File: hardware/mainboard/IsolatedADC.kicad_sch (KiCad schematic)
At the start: 22 parts, among them IC4 ADC 24bit, IC5 LTC1799

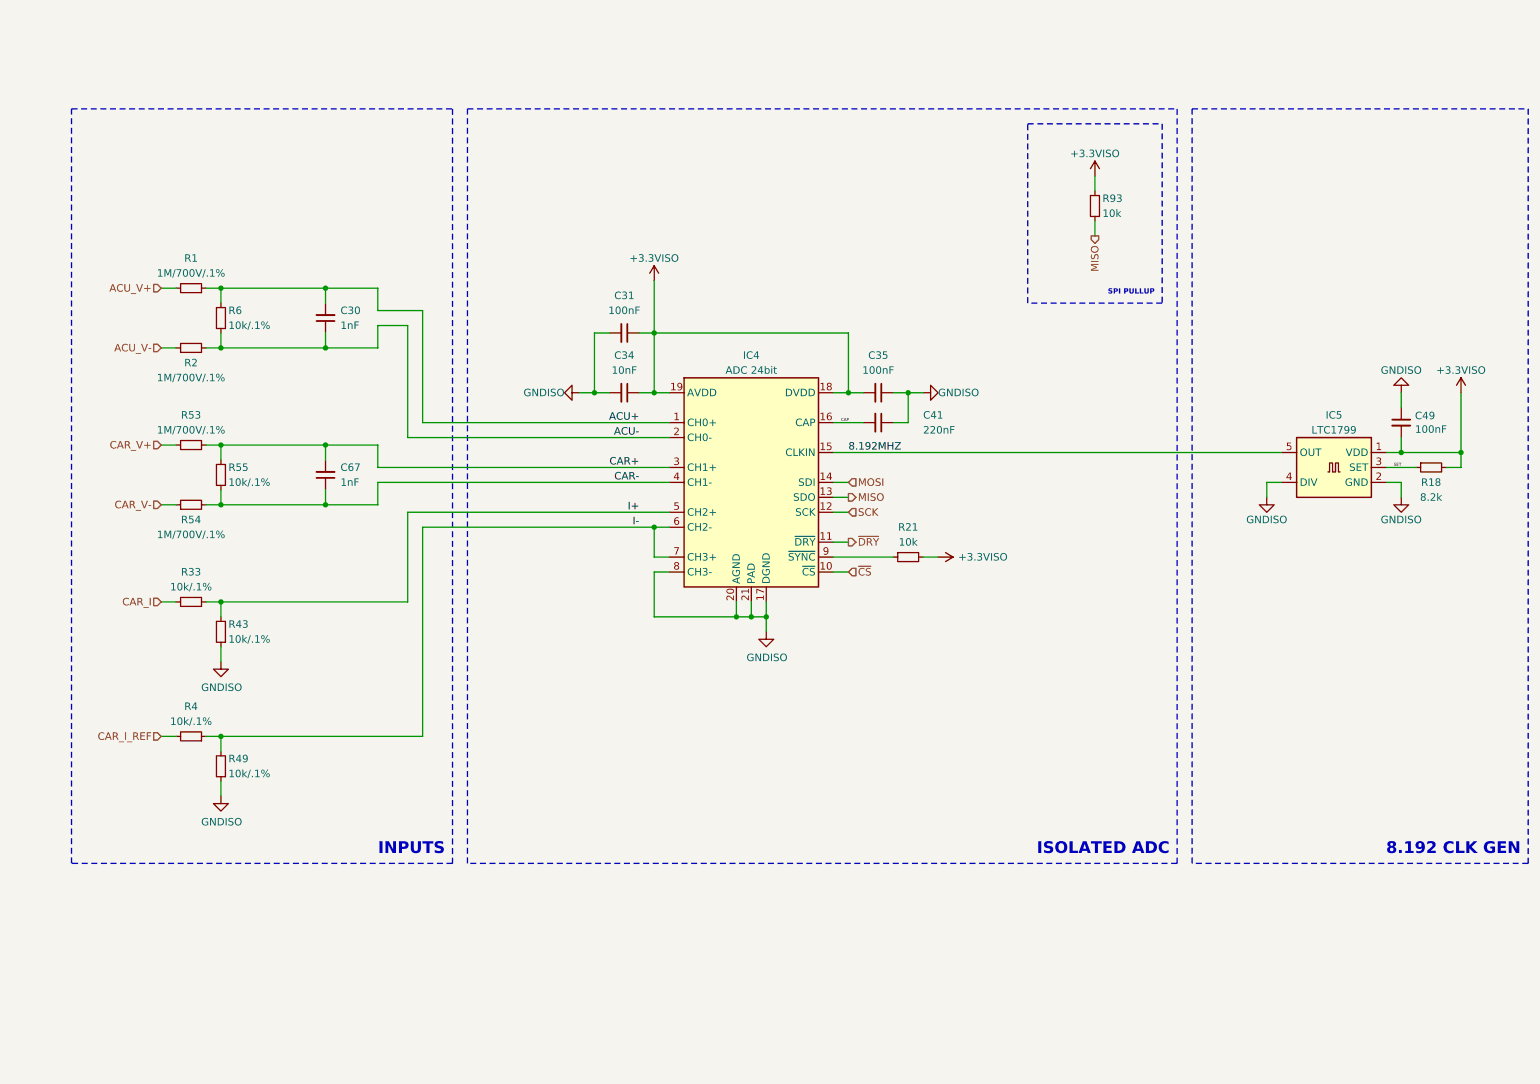
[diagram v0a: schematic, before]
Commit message: sync
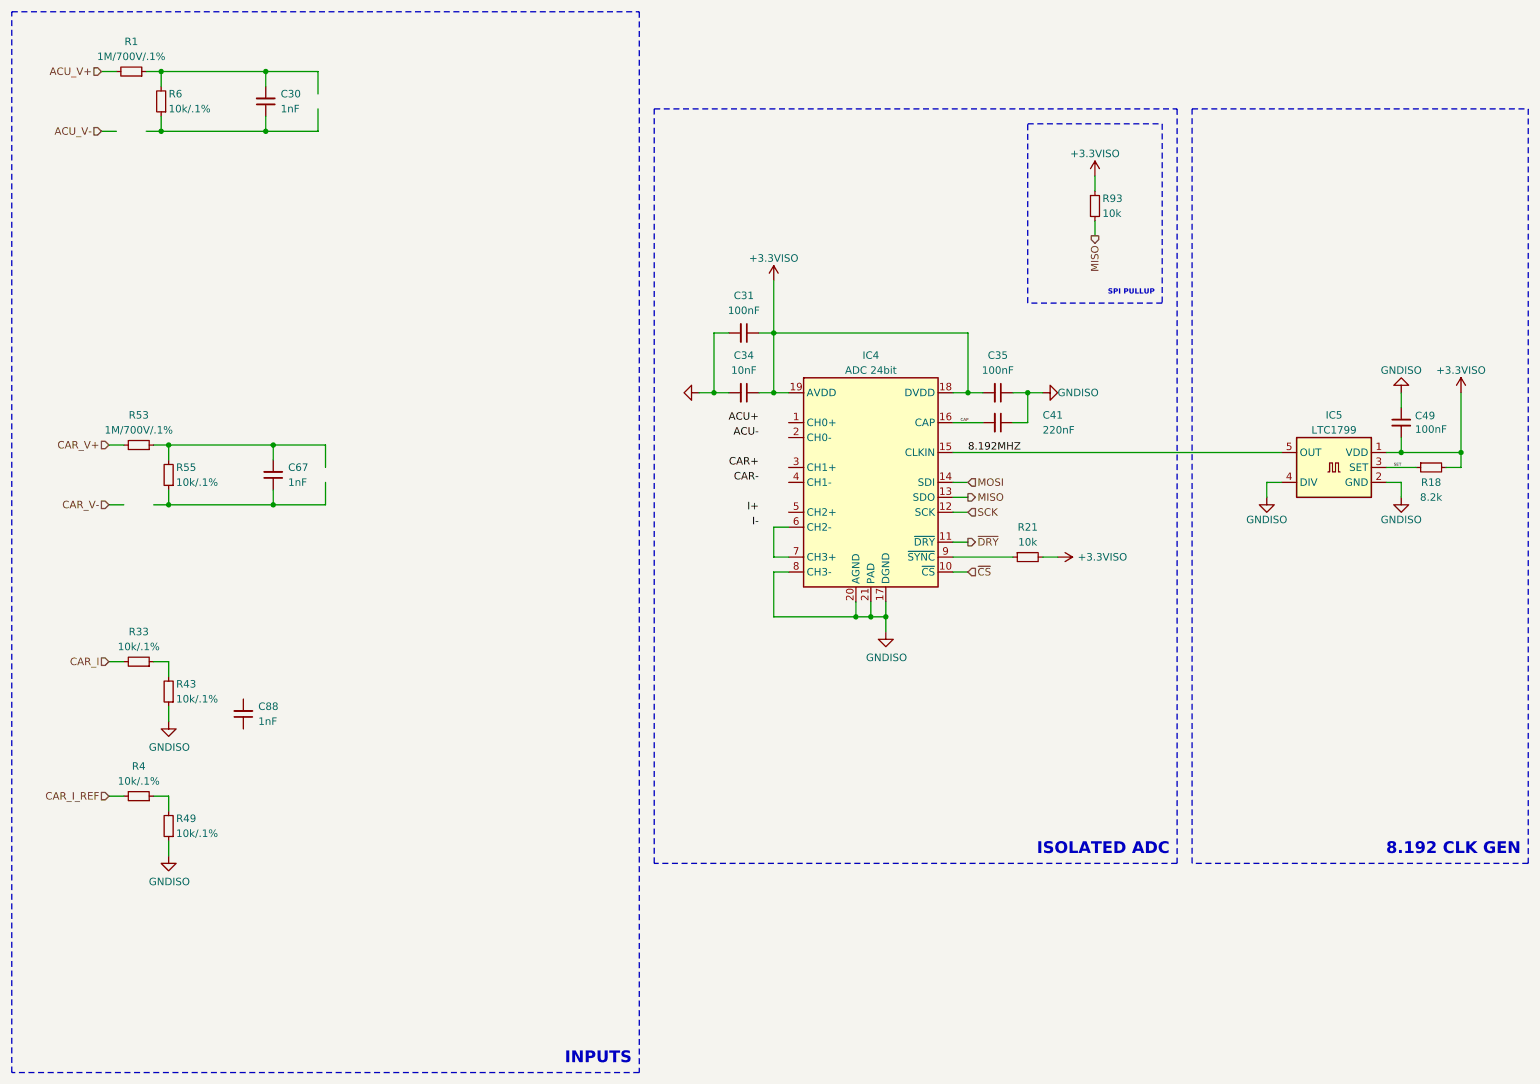
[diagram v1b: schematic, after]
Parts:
- removed R2, R54: 1M/700V/.1%, Resistor_SMD:R_1206_3216Metric, symbol Device:R_Small
- added C88: 1nF, Capacitor_SMD:C_0603_1608Metric, symbol Device:C_Small
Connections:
- net ACU+: no longer C30.2, IC4.1 (CH0+), R1.1, R6.2
- net ACU-: no longer C30.1, IC4.2 (CH0-), R6.1
- net CAR+: no longer C67.2, IC4.3 (CH1+), R53.1, R55.2
- net CAR-: no longer C67.1, IC4.4 (CH1-), R55.1
- net I+: no longer IC4.5 (CH2+), R33.1, R43.2
- net I-: no longer IC4.6 (CH2-), IC4.7 (CH3+), R4.1, R49.2
- new net: C67.1, R55.1
- new net: C67.2, R53.1, R55.2
- new net: C30.2, R1.1, R6.2
- new net: C30.1, R6.1
- new net: R4.1, R49.2
- new net: IC4.6 (CH2-), IC4.7 (CH3+)
- new net: R33.1, R43.2
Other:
- moved on the sheet: C30, C31, C34, C35, C41, C67, IC4, R1, R21, R33, R4, R43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
